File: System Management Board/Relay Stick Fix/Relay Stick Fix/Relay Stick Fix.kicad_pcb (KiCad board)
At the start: 4 copper layers, 26.8 x 30.2 mm, 13 parts, among them J1 Conn_02x04, J1 Conn_02x04_Odd_Even, J2 Castellations, J2 Structural Header, J3 Structural connector, Q1 NMOS, SW1 SW_SPDT, U1 UCC27511ADBV

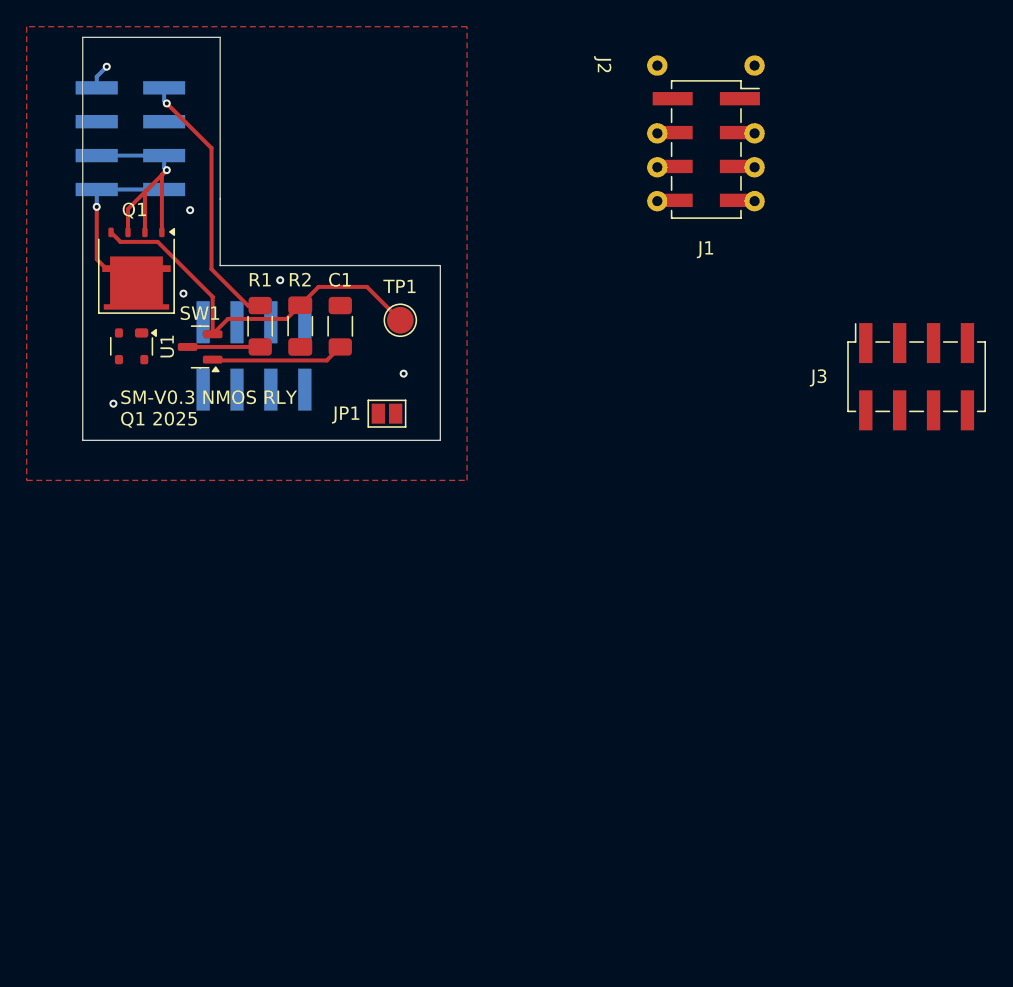
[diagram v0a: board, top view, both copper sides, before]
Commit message: before layout revision
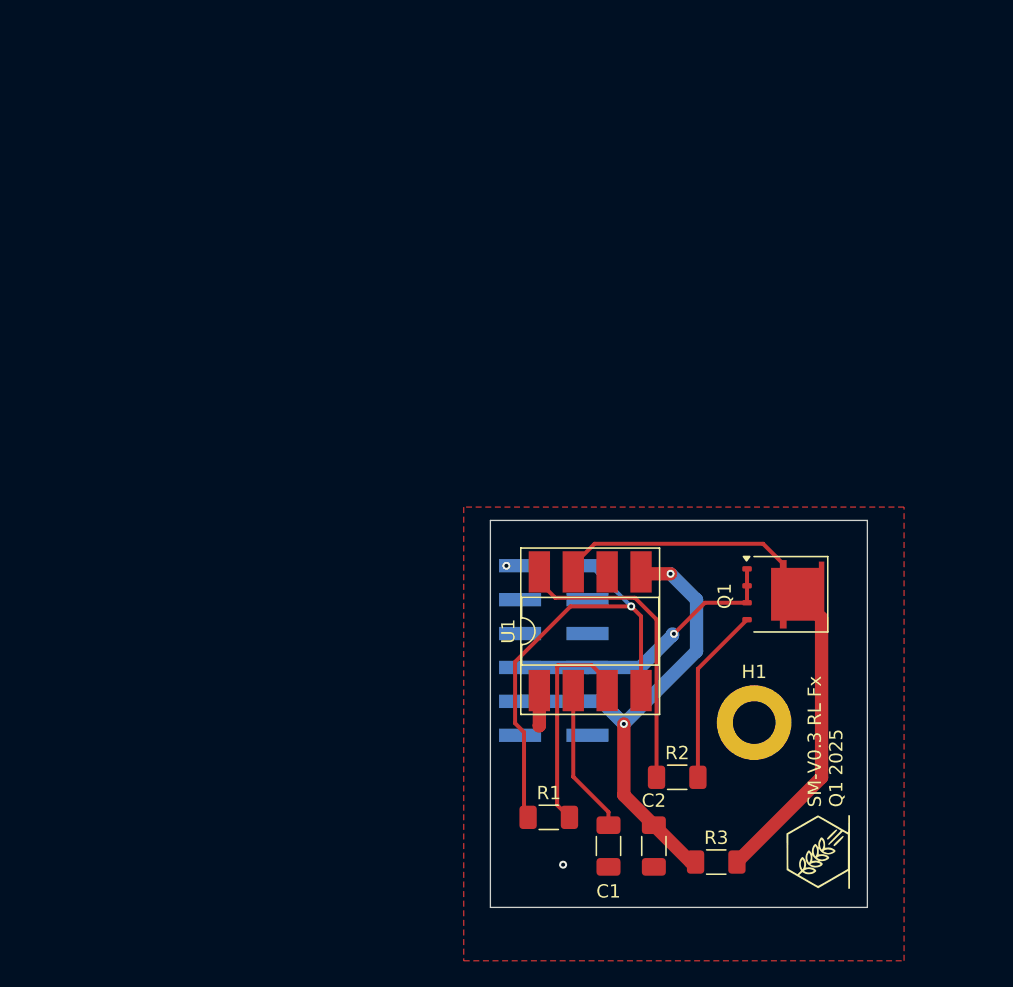
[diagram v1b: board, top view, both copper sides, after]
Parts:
- removed the J1 at (217.9, 89.2)
- removed J2: Castellations, PSA:EE2-5NU Castellated
- removed J2: Structural Header, Connector_PinHeader_2.54mm:PinHeader_2x04_P2.54mm_Vertical_SMD
- removed J3: Structural connector, Connector_PinSocket_2.54mm:PinSocket_2x04_P2.54mm_Vertical_SMD
- removed JP1: Jumper_2_Open, Jumper:SolderJumper-2_P1.3mm_Open_Pad1.0x1.5mm
- removed SW1: SW_SPDT, Package_TO_SOT_SMD:SOT-23
- removed TP1: TestPoint, TestPoint:TestPoint_Pad_D2.0mm
- added C2: 10uF, Capacitor_SMD:C_1206_3216Metric_Pad1.33x1.80mm_HandSolder, F.Cu at (214.0, 141.4)
- added H1: MountingHole_Pad, MountingHole:MountingHole_3.2mm_M3_DIN965_Pad, F.Cu at (221.5, 132.2)
- added R3: 0, Resistor_SMD:R_1206_3216Metric_Pad1.30x1.75mm_HandSolder, F.Cu at (218.7, 142.6)
- C1: value C -> 100nF
- J1: footprint Connector_PinHeader_2.54mm:PinHeader_2x04_P2.54mm_Vertical_SMD -> Connector_PinHeader_2.54mm:PinHeader_2x06_P2.54mm_Vertical_SMD
- R1: value R -> 5.1k
- R2: value R -> 0
- U1: value UCC27511ADBV -> ~; footprint Package_TO_SOT_SMD:SOT-143 -> Package_DIP:DIP-8_W8.89mm_SMDSocket_LongPads
- moved Q1 54.3 mm to (223.7, 122.5), turned to 0 degrees
- moved J1 49.8 mm to (206.5, 126.8)
- moved C1 45.3 mm to (210.6, 141.4)
- moved R1 42.7 mm to (206.1, 139.2), turned to 0 degrees
- moved R2 42.2 mm to (215.8, 136.2), turned to 0 degrees
- moved U1 40.5 mm to (209.2, 125.3), turned to 90 degrees
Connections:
- C1 pad 1: Net-(Q1-G) -> Net-(U1-TIMER)
- J1 pad 5: /i3 -> unconnected-(J1-Pin_5-Pad5)
- J1 pad 6: /i3 -> unconnected-(J1-Pin_6-Pad6)
- J1 pad 7: /Vbat Prot -> /i3
- J1 pad 8: /Vbat Prot -> /i3
- Q1 pad 5: /Vbat Prot -> Net-(Q1-D)
- R1 pad 2: Net-(SW1-C) -> /Fault
- R2 pad 1: Net-(SW1-A) -> Net-(U1-GATE)
- R2 pad 2: GND -> Net-(Q1-G)
- U1 pad 1: unconnected-(U1-V_{DD}-Pad1) -> GND
- U1 pad 2: unconnected-(U1-OUTH-Pad2) -> Net-(U1-TIMER)
- U1 pad 3: unconnected-(U1-OUTL-Pad3) -> /Fault
- U1 pad 4: unconnected-(U1-GND-Pad4) -> /5V Bootstrap
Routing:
- net Net-(Q1-D): track 0.00 -> 41.0 mm
- net /Vbat Prot: track 11.3 -> 37.8 mm, vias 1 -> 2
- net Net-(U1-GATE): track 0.00 -> 22.5 mm
- net /Fault: track 0.00 -> 16.7 mm
- net Net-(Q1-G): track 29.0 -> 13.3 mm
- net /5V Bootstrap: track 19.8 -> 33.6 mm
- net Net-(U1-TIMER): track 0.00 -> 11.2 mm
- net Net-(SW1-A): track 10.0 -> 0.00 mm
- net Net-(SW1-C): track 5.44 -> 0.00 mm
- net /i3: track 20.1 -> 21.5 mm
- net GND: track 1.89 -> 2.66 mm, vias 6 -> 2
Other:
- board size 26.8 x 30.2 mm -> 28.2 x 29 mm
- board text added: "SM-V0.3 RL Fx Q1 2025"
- board text removed: "Outline of the Castellated Layer Below"
- board text removed: "SM-V0.3 NMOS RLY Q1 2025"
